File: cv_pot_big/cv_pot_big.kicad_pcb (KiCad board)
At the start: 2 copper layers, 24 x 17 mm, 13 parts, among them J1 I/O connector, U1 HT7550-1, U2 LMV321IDBVR

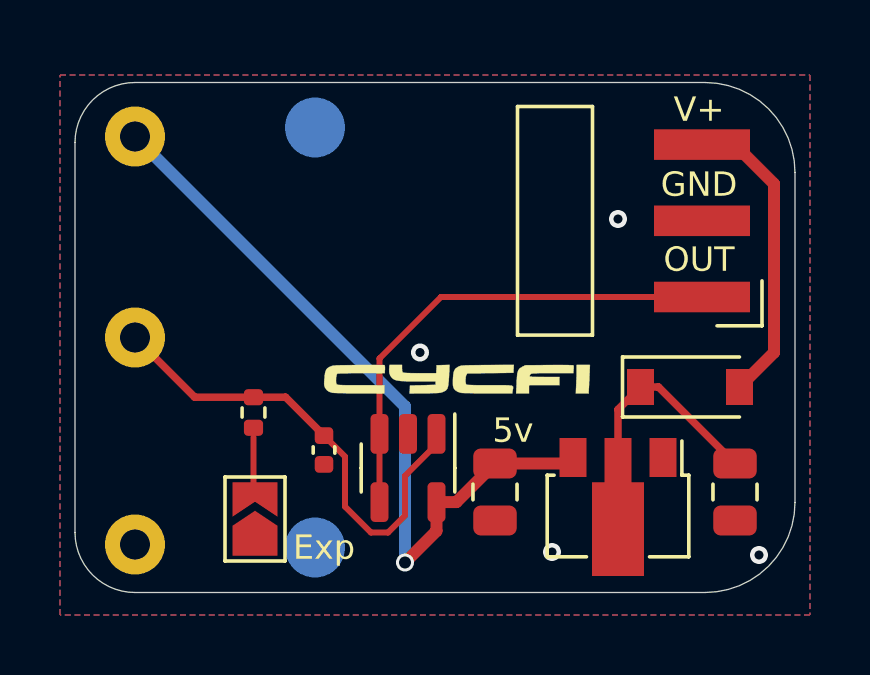
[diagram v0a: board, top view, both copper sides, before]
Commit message: refinements
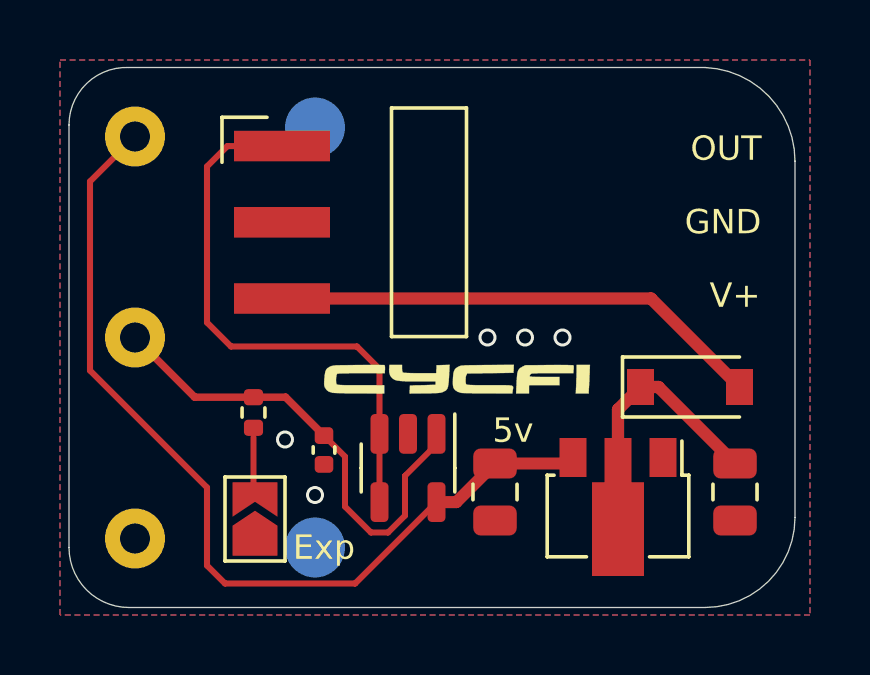
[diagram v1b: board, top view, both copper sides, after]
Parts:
- moved J1 14.9 mm to (140.9, 73.6), turned to 0 degrees
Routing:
- net V+: track 10.2 -> 16.5 mm
- net 5v: track 25.5 -> 30.7 mm, vias 1 -> 0
- net OUT: track 16.4 -> 18.8 mm
- net GND: vias 4 -> 5
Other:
- board size 24 x 17 mm -> 24.2 x 18 mm
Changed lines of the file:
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@@
     (pad "2" thru_hole circle (at 0 0) (size 2 2) (drill 1) (layers *.Cu *.Mask)
       (net 4 "/pot_center") (pinfunction "2") (pintype "passive"))
-    (pad "3" thru_hole circle (at 0 6.9) (size 2 2) (drill 1) (layers *.Cu *.Mask)
+    (pad "3" thru_hole circle (at 0 6.7) (size 2 2) (drill 1) (layers *.Cu *.Mask)
       (net 2 "GND") (pinfunction "3") (pintype "passive"))
   )
   (footprint "cycfi_library:pin_header_1x3p_2.54mm_smd_horizontal" (layer "F.Cu")
-    (at 154.9 78.65 180)
+    (at 140.9 73.62)
     (property "Sheetfile" "cv_pot_small.kicad_sch")
     (property "Sheetname" "")
@@
     (fp_line (start 20.15 -1.27) (end 20.15 6.35) (layer "F.Fab") (width 0.12))
     (fp_line (start 20.15 -1.27) (end 11.7 -1.27) (layer "F.Fab") (width 0.12))
-    (pad "1" smd rect (at 0 0 180) (size 3.2 1.02) (layers "F.Cu" "F.Paste" "F.Mask")
+    (pad "1" smd rect (at 0 0) (size 3.2 1.02) (layers "F.Cu" "F.Paste" "F.Mask")
       (net 6 "OUT") (pinfunction "P1") (pintype "passive"))
-    (pad "2" smd rect (at 0 2.54 180) (size 3.2 1.02) (layers "F.Cu" "F.Paste" "F.Mask")
+    (pad "2" smd rect (at 0 2.54) (size 3.2 1.02) (layers "F.Cu" "F.Paste" "F.Mask")
       (net 2 "GND") (pinfunction "P2") (pintype "passive"))
-    (pad "3" smd rect (at 0 5.08 180) (size 3.2 1.02) (layers "F.Cu" "F.Paste" "F.Mask")
+    (pad "3" smd rect (at 0 5.08) (size 3.2 1.02) (layers "F.Cu" "F.Paste" "F.Mask")
       (net 5 "V+") (pinfunction "P3") (pintype "passive"))
   )
@@
   (gr_line (start 136 80) (end 136 72) (layer "Dwgs.User") (width 0.1))
   (gr_circle (center 152 80) (end 164 80) (layer "Dwgs.User") (width 0.1) (fill none))
-  (gr_line (start 136 71.5) (end 155 71.5) (layer "Edge.Cuts") (width 0.0381))
-  (gr_arc (start 136 88.5) (mid 134.585786 87.914214) (end 134 86.5) (layer "Edge.Cuts") (width 0.0381))
-  (gr_line (start 158 74.5) (end 158 85.5) (layer "Edge.Cuts") (width 0.0381))
-  (gr_line (start 134 86.5) (end 134 73.5) (layer "Edge.Cuts") (width 0.0381))
-  (gr_arc (start 155 71.5) (mid 157.12132 72.37868) (end 158 74.5) (layer "Edge.Cuts") (width 0.0381))
-  (gr_arc (start 158 85.5) (mid 157.12132 87.62132) (end 155 88.5) (layer "Edge.Cuts") (width 0.0381))
-  (gr_line (start 155 88.5) (end 136 88.5) (layer "Edge.Cuts") (width 0.0381))
-  (gr_arc (start 134 73.5) (mid 134.585786 72.085786) (end 136 71.5) (layer "Edge.Cuts") (width 0.0381))
+  (gr_line (start 135.8 71) (end 155 71) (layer "Edge.Cuts") (width 0.0381))
+  (gr_arc (start 135.8 89) (mid 134.385786 88.414214) (end 133.8 87) (layer "Edge.Cuts") (width 0.0381))
+  (gr_line (start 158 74.12132) (end 158 86) (layer "Edge.Cuts") (width 0.0381))
+  (gr_line (start 133.8 87) (end 133.8 72.914214) (layer "Edge.Cuts") (width 0.0381))
+  (gr_arc (start 155 71) (mid 157.128401 71.956683) (end 158 74.12132) (layer "Edge.Cuts") (width 0.0381))
+  (gr_arc (start 158 86) (mid 157.121318 88.121318) (end 155 89) (layer "Edge.Cuts") (width 0.0381))
+  (gr_line (start 155 89) (end 135.8 89) (layer "Edge.Cuts") (width 0.0381))
+  (gr_arc (start 133.8 72.914214) (mid 134.39121 71.529997) (end 135.8 71) (layer "Edge.Cuts") (width 0.0381))
   (gr_text "Exp" (at 142.3 87) (layer "F.SilkS")
     (effects (font (size 0.8128 0.8128) (thickness 0.1524)))
@@
     (effects (font (size 0.8128 0.8128) (thickness 0.1524)))
   )
-  (gr_text "GND" (at 154.8 74.9) (layer "F.SilkS")
+  (gr_text "GND" (at 155.6 76.15) (layer "F.SilkS")
     (effects (font (size 0.8128 0.8128) (thickness 0.1524)))
   )
-  (gr_text "V+" (at 154.8 72.4) (layer "F.SilkS")
+  (gr_text "V+" (at 156 78.6) (layer "F.SilkS")
     (effects (font (size 0.8128 0.8128) (thickness 0.1524)))
   )
-  (gr_text "OUT" (at 154.8 77.4) (layer "F.SilkS")
+  (gr_text "OUT" (at 155.7 73.7) (layer "F.SilkS")
     (effects (font (size 0.8128 0.8128) (thickness 0.1524)))
   )
@@
     (effects (font (size 1 1) (thickness 0.15)))
   )
-  (segment (start 152.85 81.65) (end 152.1 82.4) (width 0.25) (layer "F.Cu") (net 1))
-  (segment (start 153.45 81.65) (end 152.85 81.65) (width 0.25) (layer "F.Cu") (net 1))
-  (segment (start 152.1 82.4) (end 152.1 84.0875) (width 0.25) (layer "F.Cu") (net 1))
-  (segment (start 156 84.2) (end 153.45 81.65) (width 0.25) (layer "F.Cu") (net 1))
-  (via (at 149.9 87.15) (size 0.6) (drill 0.3) (layers "F.Cu" "B.Cu") (free) (net 2))
-  (via (at 145.5 80.5) (size 0.6) (drill 0.3) (layers "F.Cu" "B.Cu") (free) (net 2))
-  (via (at 152.1 76.05) (size 0.6) (drill 0.3) (layers "F.Cu" "B.Cu") (free) (net 2))
-  (via (at 156.8 87.25) (size 0.6) (drill 0.3) (layers "F.Cu" "B.Cu") (free) (net 2))
-  (segment (start 146.05 85.4875) (end 146.05 86.45) (width 0.4) (layer "F.Cu") (net 3))
+  (segment (start 152.1 82.4) (end 152.1 84.0875) (width 0.4084) (layer "F.Cu") (net 1))
+  (segment (start 156 84.2) (end 153.45 81.65) (width 0.4084) (layer "F.Cu") (net 1))
+  (segment (start 153.45 81.65) (end 152.85 81.65) (width 0.4084) (layer "F.Cu") (net 1))
+  (segment (start 152.85 81.65) (end 152.1 82.4) (width 0.4084) (layer "F.Cu") (net 1))
+  (via (at 142 85.25) (size 0.6) (drill 0.4) (layers "F.Cu" "B.Cu") (free) (net 2))
+  (via (at 150.25 80) (size 0.6) (drill 0.4) (layers "F.Cu" "B.Cu") (free) (net 2))
+  (via (at 141 83.4) (size 0.6) (drill 0.4) (layers "F.Cu" "B.Cu") (free) (net 2))
+  (via (at 147.75 80) (size 0.6) (drill 0.4) (layers "F.Cu" "B.Cu") (free) (net 2))
+  (via (at 149 80) (size 0.6) (drill 0.4) (layers "F.Cu" "B.Cu") (free) (net 2))
+  (segment (start 139 88.2) (end 143.3375 88.2) (width 0.2032) (layer "F.Cu") (net 3))
   (segment (start 148 84.2) (end 150.4 84.2) (width 0.4) (layer "F.Cu") (net 3))
   (segment (start 146.05 85.4875) (end 146.7125 85.4875) (width 0.4) (layer "F.Cu") (net 3))
-  (segment (start 146.05 86.45) (end 145 87.5) (width 0.4) (layer "F.Cu") (net 3))
+  (segment (start 138.4 87.6) (end 139 88.2) (width 0.2032) (layer "F.Cu") (net 3))
+  (segment (start 134.5 81.1) (end 138.4 85) (width 0.2032) (layer "F.Cu") (net 3))
+  (segment (start 134.5 74.8) (end 134.5 81.1) (width 0.2032) (layer "F.Cu") (net 3))
+  (segment (start 138.4 85) (end 138.4 87.6) (width 0.2032) (layer "F.Cu") (net 3))
   (segment (start 150.4 84.2) (end 150.6 84) (width 0.4) (layer "F.Cu") (net 3))
+  (segment (start 143.3375 88.2) (end 146.05 85.4875) (width 0.2032) (layer "F.Cu") (net 3))
   (segment (start 146.7125 85.4875) (end 148 84.2) (width 0.4) (layer "F.Cu") (net 3))
-  (via (at 145 87.5) (size 0.6) (drill 0.4) (layers "F.Cu" "B.Cu") (net 3))
-  (segment (start 145 82.3) (end 136 73.3) (width 0.4) (layer "B.Cu") (net 3))
-  (segment (start 145 87.5) (end 145 82.3) (width 0.4) (layer "B.Cu") (net 3))
+  (segment (start 136 73.3) (end 134.5 74.8) (width 0.2032) (layer "F.Cu") (net 3))
   (segment (start 139.95 81.99) (end 137.99 81.99) (width 0.25) (layer "F.Cu") (net 4))
   (segment (start 141.02 81.99) (end 142.3 83.27) (width 0.25) (layer "F.Cu") (net 4))
@@
   (segment (start 144.435717 86.5) (end 143.864283 86.5) (width 0.2) (layer "F.Cu") (net 4))
   (segment (start 146.05 83.2125) (end 146.05 83.560717) (width 0.2) (layer "F.Cu") (net 4))
-  (segment (start 157.3 74.88) (end 157.3 80.5) (width 0.4) (layer "F.Cu") (net 5))
-  (segment (start 155.99 73.57) (end 157.3 74.88) (width 0.4) (layer "F.Cu") (net 5))
-  (segment (start 157.3 80.5) (end 156.15 81.65) (width 0.4) (layer "F.Cu") (net 5))
-  (segment (start 154.9 73.57) (end 155.99 73.57) (width 0.4) (layer "F.Cu") (net 5))
+  (segment (start 153.2 78.7) (end 140.9 78.7) (width 0.4084) (layer "F.Cu") (net 5))
+  (segment (start 156.15 81.65) (end 153.2 78.7) (width 0.4084) (layer "F.Cu") (net 5))
+  (segment (start 144.15 81.05) (end 143.4 80.3) (width 0.2032) (layer "F.Cu") (net 6))
+  (segment (start 138.4 74.3) (end 139.08 73.62) (width 0.2032) (layer "F.Cu") (net 6))
   (segment (start 144.15 85.4875) (end 144.15 83.2125) (width 0.2) (layer "F.Cu") (net 6))
-  (segment (start 144.15 80.7) (end 146.2 78.65) (width 0.2) (layer "F.Cu") (net 6))
-  (segment (start 144.15 83.2125) (end 144.15 80.7) (width 0.2) (layer "F.Cu") (net 6))
-  (segment (start 146.2 78.65) (end 154.9 78.65) (width 0.2) (layer "F.Cu") (net 6))
+  (segment (start 143.4 80.3) (end 139.2 80.3) (width 0.2032) (layer "F.Cu") (net 6))
+  (segment (start 144.15 83.2125) (end 144.15 81.05) (width 0.2032) (layer "F.Cu") (net 6))
+  (segment (start 138.4 79.5) (end 138.4 74.3) (width 0.2032) (layer "F.Cu") (net 6))
+  (segment (start 139.08 73.62) (end 140.9 73.62) (width 0.2032) (layer "F.Cu") (net 6))
+  (segment (start 139.2 80.3) (end 138.4 79.5) (width 0.2032) (layer "F.Cu") (net 6))
   (segment (start 139.95 85.275) (end 140 85.325) (width 0.2) (layer "F.Cu") (net 7))
   (segment (start 139.95 83.325) (end 139.95 85.275) (width 0.2) (layer "F.Cu") (net 7))
@@
         (xy 158.5 89.25)
         (xy 133.5 89.25)
-        (xy 133.5 71.25)
-        (xy 158.5 71.25)
+        (xy 133.5 70.75)
+        (xy 158.5 70.75)
       )
     )
@@
         (xy 158.5 89.25)
         (xy 133.5 89.25)
-        (xy 133.5 71.25)
-        (xy 158.5 71.25)
+        (xy 133.5 70.75)
+        (xy 158.5 70.75)
       )
     )
